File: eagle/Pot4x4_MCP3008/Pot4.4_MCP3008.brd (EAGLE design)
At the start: 70.8 x 45.7 mm, 17 parts, among them IC1 MCP3008, IC2 MCP3008

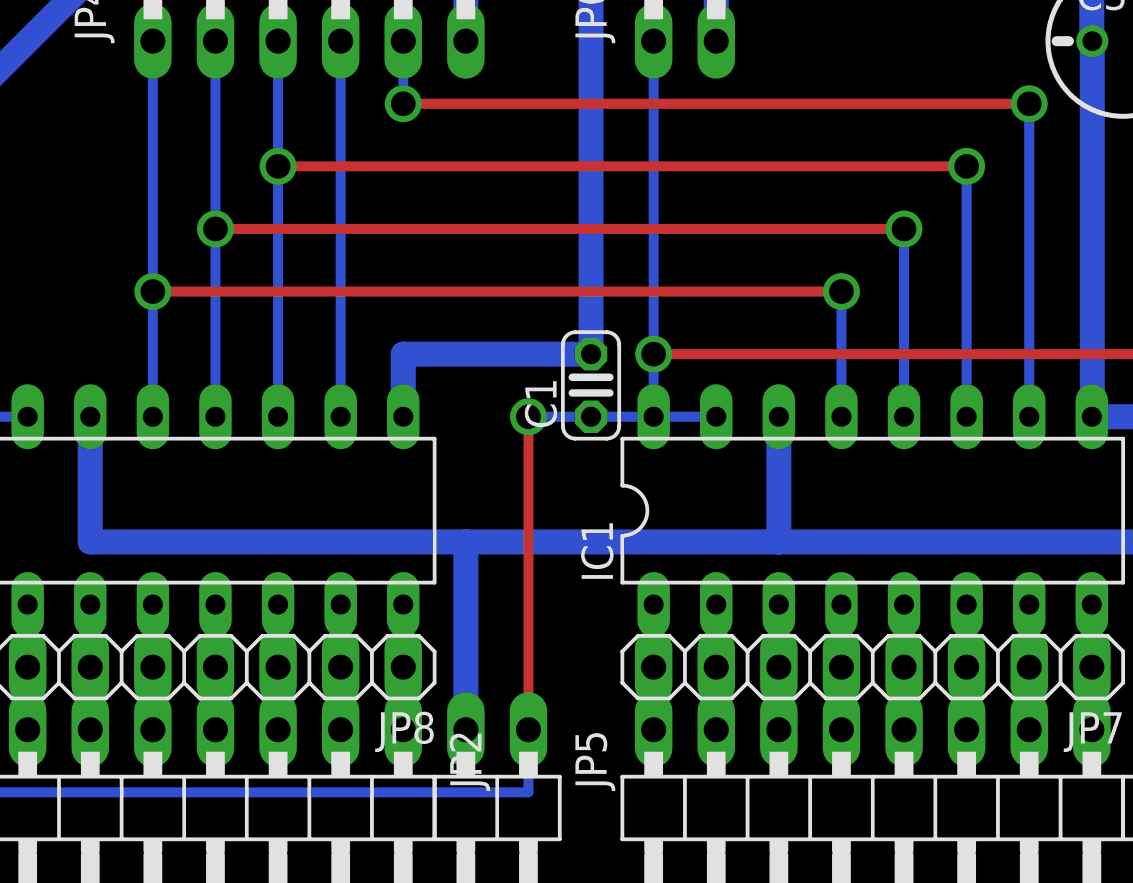
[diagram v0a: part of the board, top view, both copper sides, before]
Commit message: update
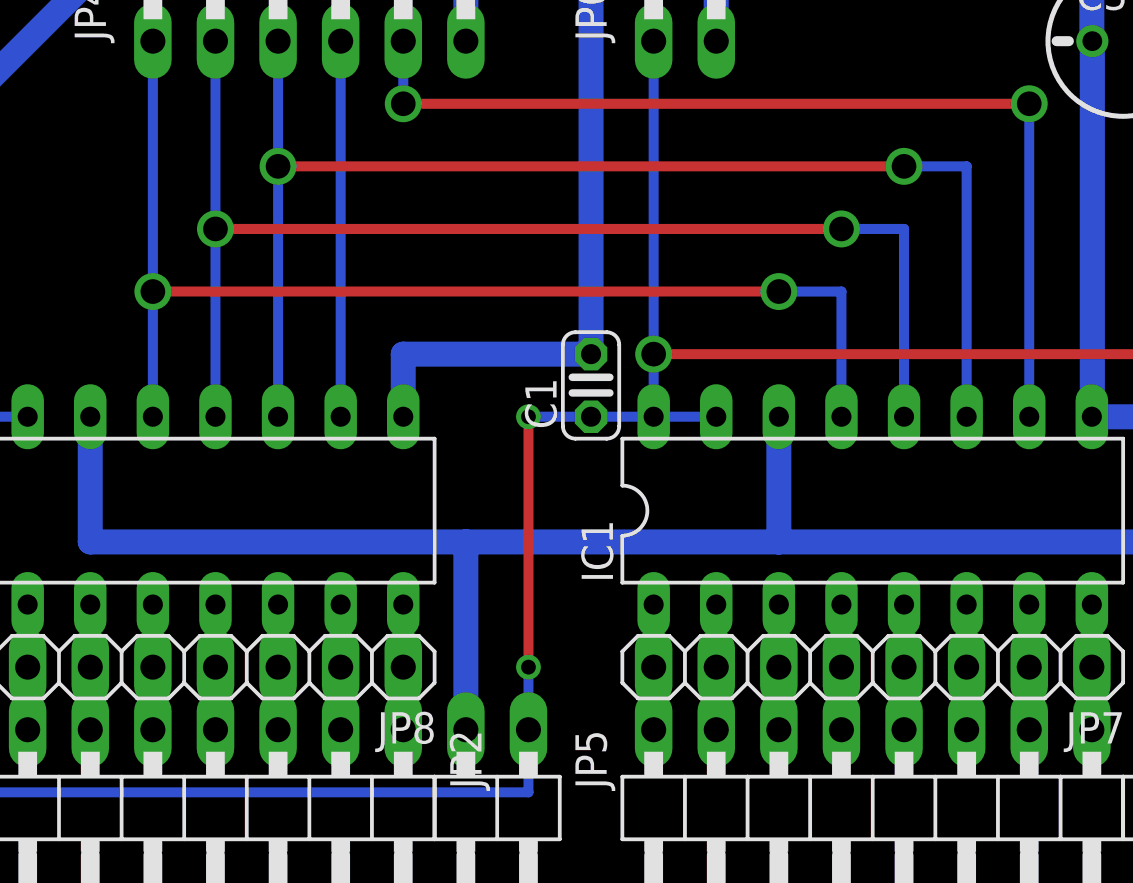
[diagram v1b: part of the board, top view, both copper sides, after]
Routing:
- net +5V: vias 3 -> 4
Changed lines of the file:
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@@
 <wire x1="38.1" y1="38.1" x2="38.1" y2="25.4" width="0.4064" layer="16"/>
 <wire x1="38.1" y1="25.4" x2="38.1" y2="22.86" width="0.4064" layer="16"/>
-<wire x1="33.02" y1="22.86" x2="33.02" y2="10.16" width="0.4064" layer="1"/>
-<via x="33.02" y="22.86" extent="1-16" drill="1" shape="square"/>
 <wire x1="40.64" y1="22.86" x2="38.1" y2="22.86" width="0.4064" layer="16"/>
 <wire x1="60.96" y1="10.16" x2="60.96" y2="25.4" width="0.4064" layer="16"/>
@@
 <contactref element="LED1" pad="A"/>
 <wire x1="60.96" y1="27.94" x2="60.96" y2="25.4" width="0.4064" layer="16"/>
+<wire x1="33.02" y1="22.86" x2="33.02" y2="12.7" width="0.4064" layer="1"/>
+<via x="33.02" y="22.86" extent="1-16" drill="0.6" shape="square"/>
+<via x="33.02" y="12.7" extent="1-16" drill="0.6" shape="square"/>
+<wire x1="33.02" y1="12.7" x2="33.02" y2="10.16" width="0.4064" layer="16"/>
 </signal>
 <signal name="AGND">
@@
 <contactref element="IC2" pad="13"/>
 <wire x1="17.78" y1="27.94" x2="17.78" y2="22.86" width="0.4064" layer="16"/>
-<wire x1="45.72" y1="22.86" x2="45.72" y2="27.94" width="0.4064" layer="16"/>
-<wire x1="45.72" y1="27.94" x2="17.78" y2="27.94" width="0.4064" layer="1"/>
-<via x="45.72" y="27.94" extent="1-16" drill="1" shape="square"/>
+<wire x1="43.18" y1="27.94" x2="17.78" y2="27.94" width="0.4064" layer="1"/>
+<via x="43.18" y="27.94" extent="1-16" drill="1" shape="square"/>
 <via x="17.78" y="27.94" extent="1-16" drill="1" shape="square"/>
 <contactref element="JP4" pad="1"/>
 <wire x1="17.78" y1="38.1" x2="17.78" y2="27.94" width="0.4064" layer="16"/>
+<wire x1="45.72" y1="22.86" x2="45.72" y2="27.94" width="0.4064" layer="16"/>
+<wire x1="45.72" y1="27.94" x2="43.18" y2="27.94" width="0.4064" layer="16"/>
 </signal>
 <signal name="MISO">
@@
 <contactref element="IC2" pad="12"/>
 <wire x1="20.32" y1="30.48" x2="20.32" y2="22.86" width="0.4064" layer="16"/>
-<wire x1="48.26" y1="22.86" x2="48.26" y2="30.48" width="0.4064" layer="16"/>
-<wire x1="48.26" y1="30.48" x2="20.32" y2="30.48" width="0.4064" layer="1"/>
-<via x="48.26" y="30.48" extent="1-16" drill="1" shape="square"/>
+<wire x1="45.72" y1="30.48" x2="20.32" y2="30.48" width="0.4064" layer="1"/>
+<via x="45.72" y="30.48" extent="1-16" drill="1" shape="square"/>
 <via x="20.32" y="30.48" extent="1-16" drill="1" shape="square"/>
 <contactref element="JP4" pad="2"/>
 <wire x1="20.32" y1="38.1" x2="20.32" y2="30.48" width="0.4064" layer="16"/>
+<wire x1="48.26" y1="22.86" x2="48.26" y2="30.48" width="0.4064" layer="16"/>
+<wire x1="48.26" y1="30.48" x2="45.72" y2="30.48" width="0.4064" layer="16"/>
 </signal>
 <signal name="MOSI">
@@
 <contactref element="IC1" pad="11"/>
 <wire x1="22.86" y1="33.02" x2="22.86" y2="22.86" width="0.4064" layer="16"/>
-<wire x1="50.8" y1="22.86" x2="50.8" y2="33.02" width="0.4064" layer="16"/>
-<wire x1="50.8" y1="33.02" x2="22.86" y2="33.02" width="0.4064" layer="1"/>
-<via x="50.8" y="33.02" extent="1-16" drill="1" shape="square"/>
+<wire x1="48.26" y1="33.02" x2="22.86" y2="33.02" width="0.4064" layer="1"/>
+<via x="48.26" y="33.02" extent="1-16" drill="1" shape="square"/>
 <via x="22.86" y="33.02" extent="1-16" drill="1" shape="square"/>
 <contactref element="JP4" pad="3"/>
 <wire x1="22.86" y1="38.1" x2="22.86" y2="33.02" width="0.4064" layer="16"/>
+<wire x1="50.8" y1="22.86" x2="50.8" y2="33.02" width="0.4064" layer="16"/>
+<wire x1="50.8" y1="33.02" x2="48.26" y2="33.02" width="0.4064" layer="16"/>
 </signal>
 <signal name="GND">
